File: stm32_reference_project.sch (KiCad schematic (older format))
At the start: 37 parts, among them J1 USB_Serial, J2 PROG_HDR, SW1 RESET, SW2 BOOT_SELECT, SW3 BAT_SELECT, U1 AMS1117-3.3, U2 STM32F103C8Tx, Y1 8Mhz, Y2 32.768K

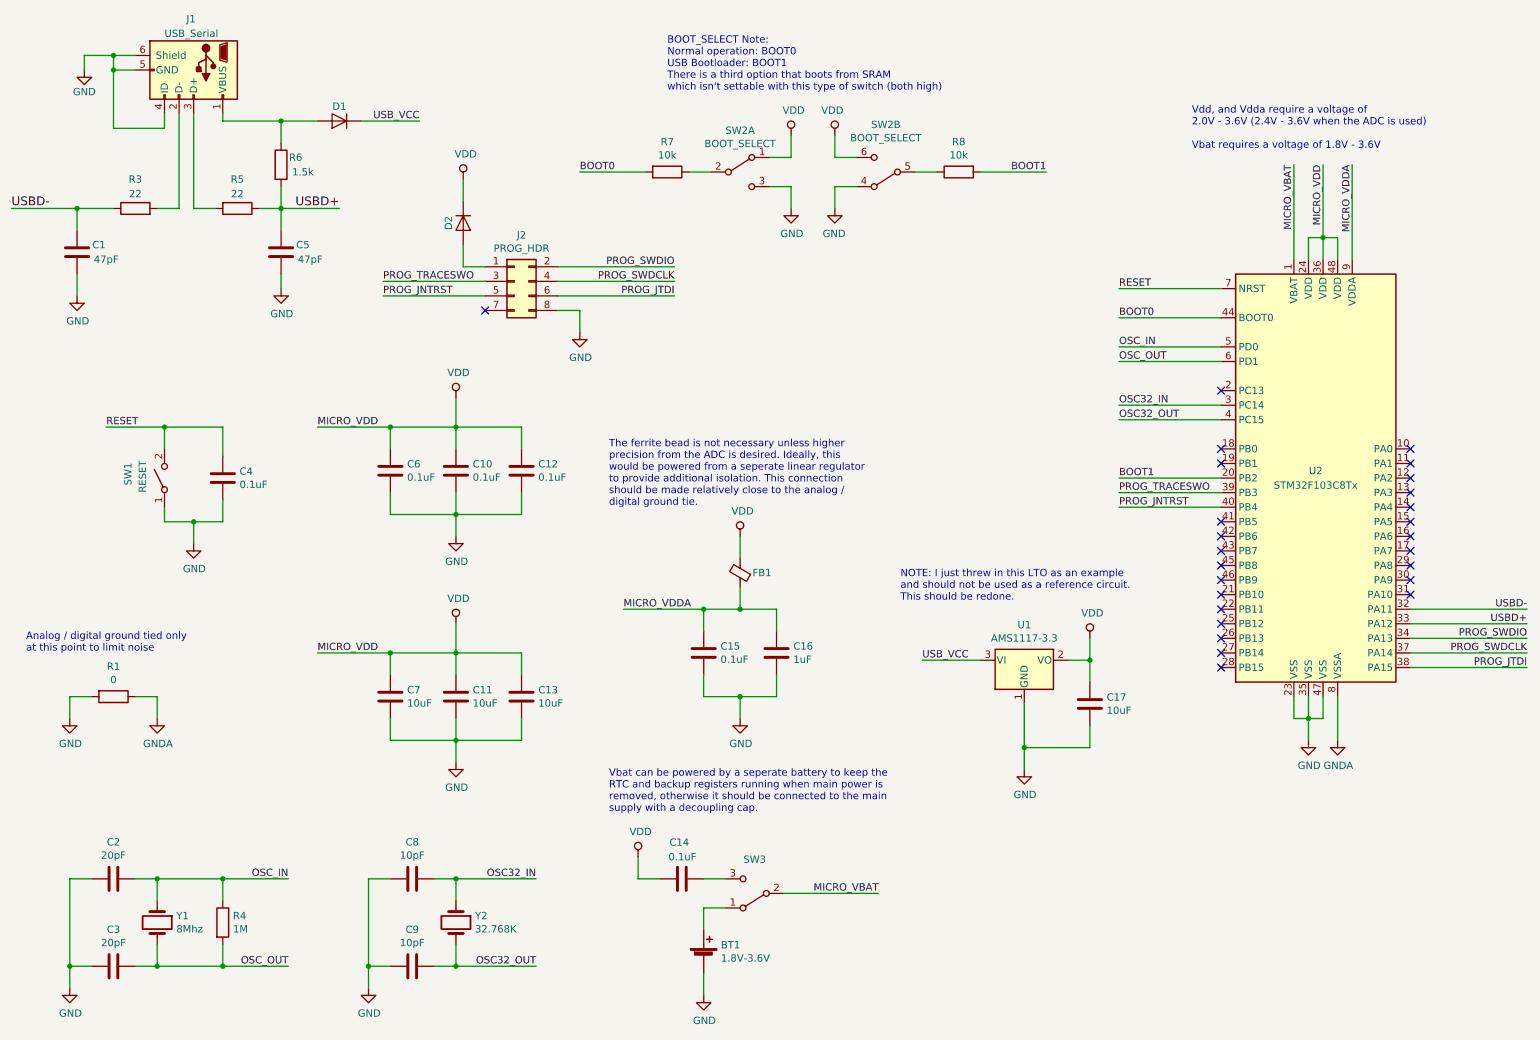
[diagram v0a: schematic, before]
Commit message: A drunken cleanup
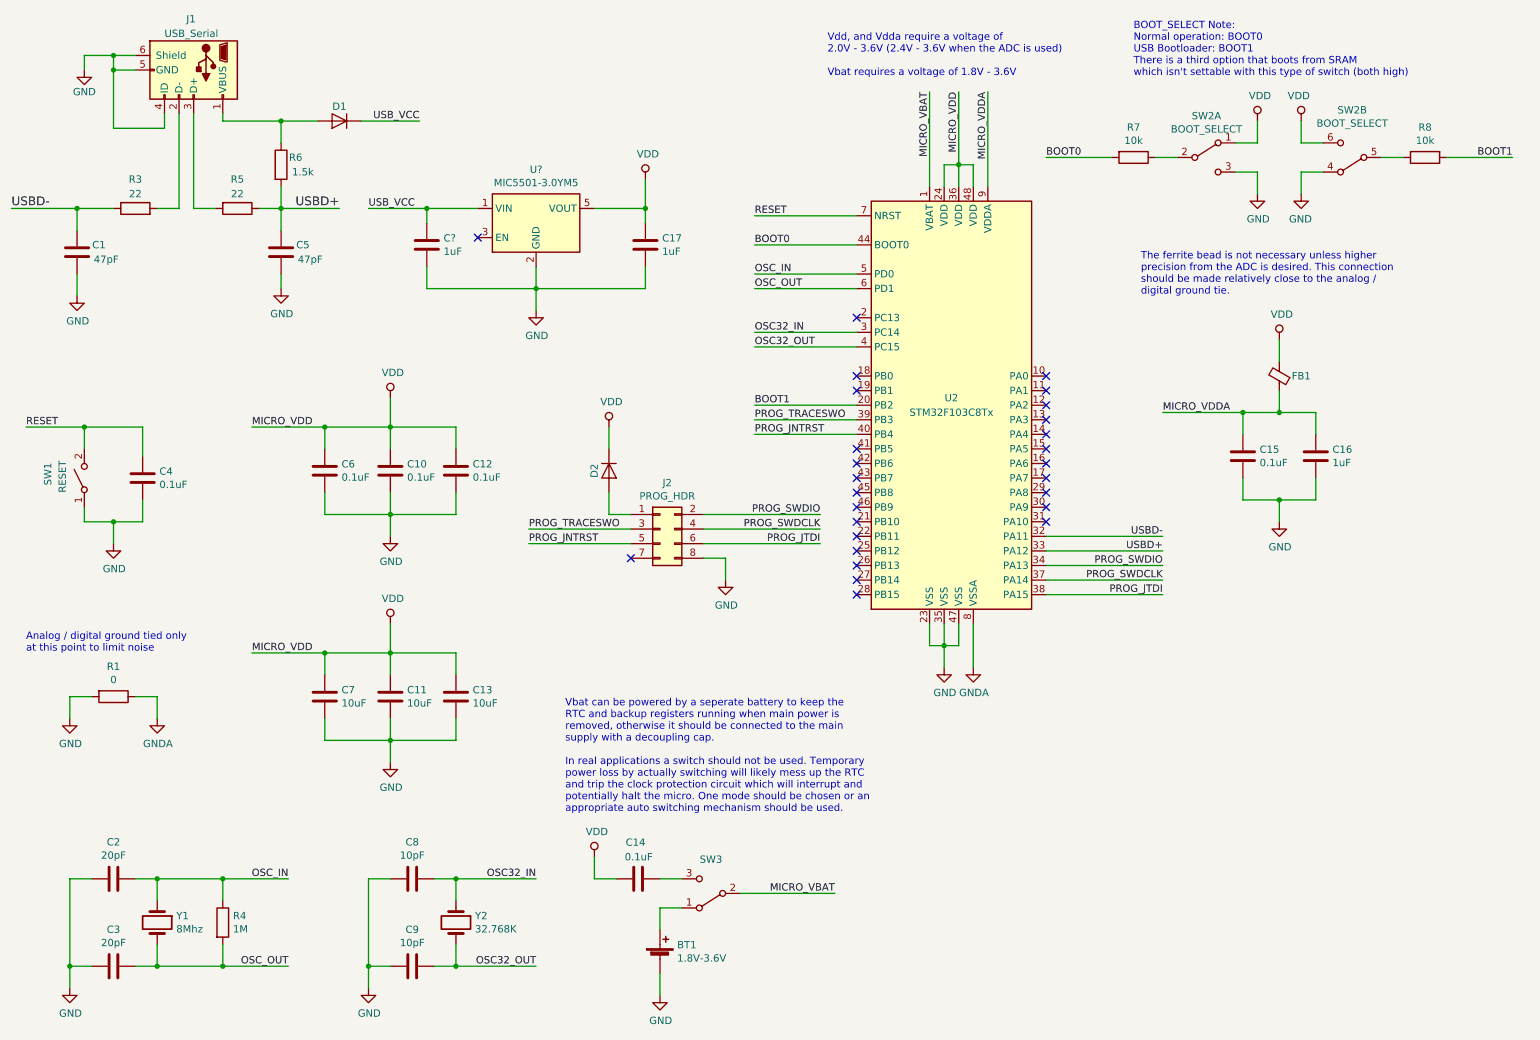
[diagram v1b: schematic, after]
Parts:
- removed U1: AMS1117-3.3, Package_TO_SOT_SMD:SOT-223-3_TabPin2, symbol Regulator_Linear:AMS1117-3.3
- added C?: 1uF, Capacitor_SMD:C_0603_1608Metric, symbol Device:C
- added U?: MIC5501-3.0YM5, Package_TO_SOT_SMD:SOT-23-5, symbol Regulator_Linear:MIC5501-3.0YM5
- C17: value 10uF -> 1uF; Spice_Model 10u -> 1u
- J1: DigiKey Part (none) -> WM11263CT-ND; DigiKey Price (none) -> 0.92
- R1: footprint Resistor_SMD:R_0603_1608Metric -> Resistor_SMD:R_0402_1005Metric; Comment (none) -> DNP / Do Not Populate
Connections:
- net GND: now also C?.2, U?.2 (GND)
- net USB_VCC: now also C?.1, U?.1 (VIN)
- net VDD: now also U?.5 (VOUT)
- no-connect marks 26 -> 27
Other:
- note added: "The ferrite bead is not necessary unless higher\nprecision from the ADC is desired. This connection\nshould be made relatively close to the analog /\ndigital ground tie."
- note added: "Vbat can be powered by a seperate battery to keep the\nRTC and backup registers running when main power is\nremoved, otherwise it should be connected to the main\nsupply with a decoupling cap.\n\nIn real applications a switch should not be used. Temporary\npower loss by actually switching will likely mess up the RTC\nand trip the clock protection circuit which will interrupt and\npotentially halt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"
- note removed: "NOTE: I just threw in this LTO as an example\nand should not be used as a reference circuit.\nThis should be redone."
- note removed: "The ferrite bead is not necessary unless higher\nprecision from the ADC is desired. Ideally, this\nwould be powered from a seperate linear regulator\nto provide additional isolation. This connection\nshould be made relatively close to the analog /\ndigital ground tie."
- note removed: "Vbat can be powered by a seperate battery to keep the\nRTC and backup registers running when main power is\nremoved, otherwise it should be connected to the main\nsupply with a decoupling cap."
- moved on the sheet: BT1, C10, C11, C12, C13, C14, C15, C16, C17, C4, C6, C7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
